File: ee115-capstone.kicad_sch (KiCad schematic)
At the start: 24 parts, among them J2 9V_BATTERY, J5 Conn_01x03_Pin, J6 Conn_02x02_Odd_Even, Q1 PMOS, Q2 NMOS, SW3 SW_Push, SW4 GF-123-0054, U13 LD39150DT33-R

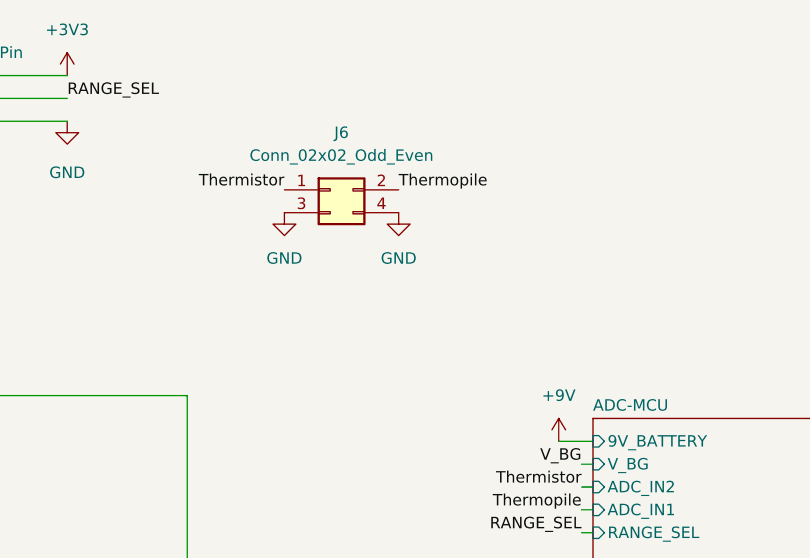
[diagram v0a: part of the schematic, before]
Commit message: init pcb
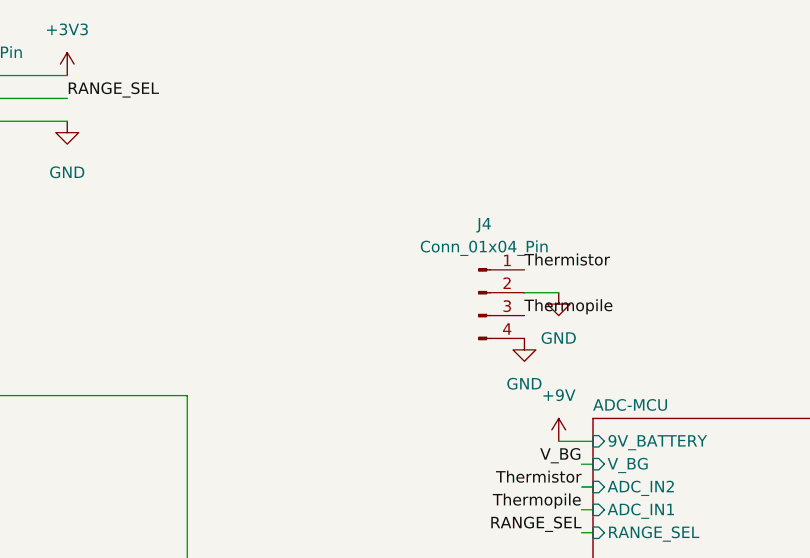
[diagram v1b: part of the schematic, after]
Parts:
- removed J6: Conn_02x02_Odd_Even, Connector_Molex:Molex_Mega-Fit_76829-0004_2x02_P5.70mm_Vertical, symbol Connector_Generic:Conn_02x02_Odd_Even
- added J4: Conn_01x04_Pin, Connector_Molex:Molex_KK-254_AE-6410-04A_1x04_P2.54mm_Vertical, symbol Connector:Conn_01x04_Pin
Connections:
- net GND: now also J4.2 (Pin_2), J4.4 (Pin_4)
- net Thermistor: now also J4.1 (Pin_1)
- net Thermopile: now also J4.3 (Pin_3)
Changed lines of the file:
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@@
+	(wire
+		(pts
+			(xy 185.42 45.72) (xy 189.23 45.72)
+		)
+		(stroke
+			(width 0)
+			(type default)
+		)
+	)
 	(wire
 		(pts
@@
 		)
 	)
+	(label "Thermopile"
+		(at 185.42 48.26 0)
+		(effects
+			(font
+				(size 1.27 1.27)
+			)
+			(justify left bottom)
+		)
+	)
 	(label "V_BG"
 		(at 191.77 64.77 180)
@@
 		)
 	)
-	(label "Thermistor"
-		(at 158.75 34.29 180)
-		(effects
-			(font
-				(size 1.27 1.27)
-			)
-			(justify right bottom)
-		)
-	)
 	(label "Thermopile"
 		(at 189.23 107.95 180)
@@
 		)
 	)
-	(label "Thermopile"
-		(at 171.45 34.29 0)
-		(effects
-			(font
-				(size 1.27 1.27)
-			)
-			(justify left bottom)
-		)
-	)
 	(label "POWER_LATCH"
 		(at 71.12 95.25 0)
@@
 		)
 	)
+	(label "Thermistor"
+		(at 185.42 43.18 0)
+		(effects
+			(font
+				(size 1.27 1.27)
+			)
+			(justify left bottom)
+		)
+	)
 	(label "Thermopile"
 		(at 191.77 69.85 180)
@@
 	)
 	(symbol
-		(lib_id "Connector_Generic:Conn_02x02_Odd_Even")
-		(at 163.83 34.29 0)
-		(unit 1)
-		(exclude_from_sim no)
-		(in_bom yes)
-		(on_board yes)
-		(dnp no)
-		(fields_autoplaced yes)
-		(property "Reference" "J6"
-			(at 165.1 27.94 0)
-			(effects
-				(font
-					(size 1.27 1.27)
-				)
-			)
-		)
-		(property "Value" "Conn_02x02_Odd_Even"
-			(at 165.1 30.48 0)
-			(effects
-				(font
-					(size 1.27 1.27)
-				)
-			)
-		)
-		(property "Footprint" "Connector_Molex:Molex_Mega-Fit_76829-0004_2x02_P5.70mm_Vertical"
-			(at 163.83 34.29 0)
-			(effects
-				(font
-					(size 1.27 1.27)
-				)
-				(hide yes)
-			)
-		)
-		(property "Datasheet" "~"
-			(at 163.83 34.29 0)
-			(effects
-				(font
-					(size 1.27 1.27)
-				)
-				(hide yes)
-			)
-		)
-		(property "Description" "Generic connector, double row, 02x02, odd/even pin numbering scheme (row 1 odd numbers, row 2 even numbers), script generated (kicad-library-utils/schlib/autogen/connector/)"
-			(at 163.83 34.29 0)
-			(effects
-				(font
-					(size 1.27 1.27)
-				)
-				(hide yes)
-			)
-		)
-		(pin "1"
-		)
-		(pin "4"
-		)
-		(pin "2"
-		)
-		(pin "3"
-		)
-		(instances
-			(project ""
-				(path "/80dfed98-7d85-4c9a-bb85-182165e7352f"
-					(reference "J6")
-					(unit 1)
-				)
-			)
-		)
-	)
-	(symbol
 		(lib_id "Connector:TestPoint")
 		(at 33.655 82.55 0)
@@
 	)
 	(symbol
+		(lib_id "power:GND")
+		(at 189.23 45.72 0)
+		(unit 1)
+		(exclude_from_sim no)
+		(in_bom yes)
+		(on_board yes)
+		(dnp no)
+		(fields_autoplaced yes)
+		(property "Reference" "#PWR0122"
+			(at 189.23 52.07 0)
+			(effects
+				(font
+					(size 1.27 1.27)
+				)
+				(hide yes)
+			)
+		)
+		(property "Value" "GND"
+			(at 189.23 50.8 0)
+			(effects
+				(font
+					(size 1.27 1.27)
+				)
+			)
+		)
+		(property "Footprint" ""
+			(at 189.23 45.72 0)
+			(effects
+				(font
+					(size 1.27 1.27)
+				)
+				(hide yes)
+			)
+		)
+		(property "Datasheet" ""
+			(at 189.23 45.72 0)
+			(effects
+				(font
+					(size 1.27 1.27)
+				)
+				(hide yes)
+			)
+		)
+		(property "Description" "Power symbol creates a global label with name \"GND\" , ground"
+			(at 189.23 45.72 0)
+			(effects
+				(font
+					(size 1.27 1.27)
+				)
+				(hide yes)
+			)
+		)
+		(pin "1"
+		)
+		(instances
+			(project "ee115-capstone"
+				(path "/80dfed98-7d85-4c9a-bb85-182165e7352f"
+					(reference "#PWR0122")
+					(unit 1)
+				)
+			)
+		)
+	)
+	(symbol
 		(lib_id "Device:C")
 		(at 90.17 60.96 0)
@@
 				(path "/80dfed98-7d85-4c9a-bb85-182165e7352f"
 					(reference "#PWR0120")
-					(unit 1)
-				)
-			)
-		)
-	)
-	(symbol
-		(lib_id "power:GND")
-		(at 158.75 36.83 0)
-		(unit 1)
-		(exclude_from_sim no)
-		(in_bom yes)
-		(on_board yes)
-		(dnp no)
-		(fields_autoplaced yes)
-		(property "Reference" "#PWR0104"
-			(at 158.75 43.18 0)
-			(effects
-				(font
-					(size 1.27 1.27)
-				)
-				(hide yes)
-			)
-		)
-		(property "Value" "GND"
-			(at 158.75 41.91 0)
-			(effects
-				(font
-					(size 1.27 1.27)
-				)
-			)
-		)
-		(property "Footprint" ""
-			(at 158.75 36.83 0)
-			(effects
-				(font
-					(size 1.27 1.27)
-				)
-				(hide yes)
-			)
-		)
-		(property "Datasheet" ""
-			(at 158.75 36.83 0)
-			(effects
-				(font
-					(size 1.27 1.27)
-				)
-				(hide yes)
-			)
-		)
-		(property "Description" "Power symbol creates a global label with name \"GND\" , ground"
-			(at 158.75 36.83 0)
-			(effects
-				(font
-					(size 1.27 1.27)
-				)
-				(hide yes)
-			)
-		)
-		(pin "1"
-		)
-		(instances
-			(project "ee115-capstone"
-				(path "/80dfed98-7d85-4c9a-bb85-182165e7352f"
-					(reference "#PWR0104")
 					(unit 1)
 				)
@@
 	(symbol
 		(lib_id "power:GND")
-		(at 171.45 36.83 0)
+		(at 185.42 50.8 0)
 		(unit 1)
 		(exclude_from_sim no)
@@
 		(fields_autoplaced yes)
 		(property "Reference" "#PWR0103"
-			(at 171.45 43.18 0)
+			(at 185.42 57.15 0)
 			(effects
 				(font
@@
 		)
 		(property "Value" "GND"
-			(at 171.45 41.91 0)
+			(at 185.42 55.88 0)
 			(effects
 				(font
@@
 		)
 		(property "Footprint" ""
-			(at 171.45 36.83 0)
+			(at 185.42 50.8 0)
 			(effects
 				(font
@@
 		)
 		(property "Datasheet" ""
-			(at 171.45 36.83 0)
+			(at 185.42 50.8 0)
 			(effects
 				(font
@@
 		)
 		(property "Description" "Power symbol creates a global label with name \"GND\" , ground"
-			(at 171.45 36.83 0)
+			(at 185.42 50.8 0)
 			(effects
 				(font
@@
 					(unit 1)
 				)
+			)
+		)
+	)
+	(symbol
+		(lib_id "Connector:Conn_01x04_Pin")
+		(at 180.34 45.72 0)
+		(unit 1)
+		(exclude_from_sim no)
+		(in_bom yes)
+		(on_board yes)
+		(dnp no)
+		(fields_autoplaced yes)
+		(property "Reference" "J4"
+			(at 180.975 38.1 0)
+			(effects
+				(font
+					(size 1.27 1.27)
+				)
+			)
+		)
+		(property "Value" "Conn_01x04_Pin"
+			(at 180.975 40.64 0)
+			(effects
+				(font
+					(size 1.27 1.27)
+				)
+			)
+		)
+		(property "Footprint" "Connector_Molex:Molex_KK-254_AE-6410-04A_1x04_P2.54mm_Vertical"
+			(at 180.34 45.72 0)
+			(effects
+				(font
+					(size 1.27 1.27)
+				)
+				(hide yes)
+			)
+		)
+		(property "Datasheet" "~"
+			(at 180.34 45.72 0)
+			(effects
+				(font
+					(size 1.27 1.27)
+				)
+				(hide yes)
+			)
+		)
+		(property "Description" "Generic connector, single row, 01x04, script generated"
+			(at 180.34 45.72 0)
+			(effects
+				(font
+					(size 1.27 1.27)
+				)
+				(hide yes)
+			)
+		)
+		(pin "1"
+		)
+		(pin "2"
+		)
+		(pin "3"
+		)
+		(pin "4"
+		)
+		(instances
+			(project ""
+				(path "/80dfed98-7d85-4c9a-bb85-182165e7352f"
+					(reference "J4")
+					(unit 1)
+				)
